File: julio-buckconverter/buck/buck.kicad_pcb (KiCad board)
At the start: 2 copper layers, 63.5 x 95.5 mm, 27 parts, among them J1 Screw_Terminal_01x02, J2 Screw_Terminal_01x02, J3 Screw_Terminal_01x02, Q1 BD911, Q2 MJE15031, U2 TL494

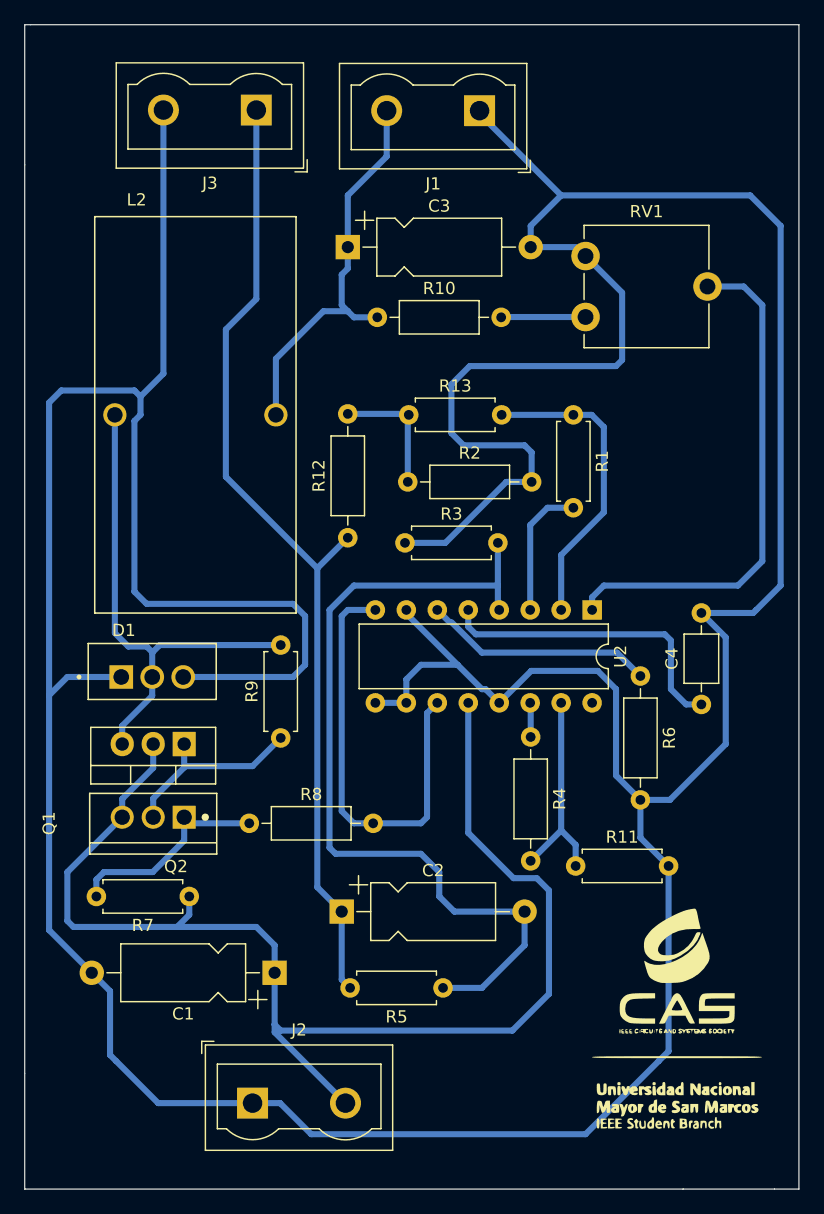
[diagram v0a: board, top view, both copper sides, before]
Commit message: CASI FINAL
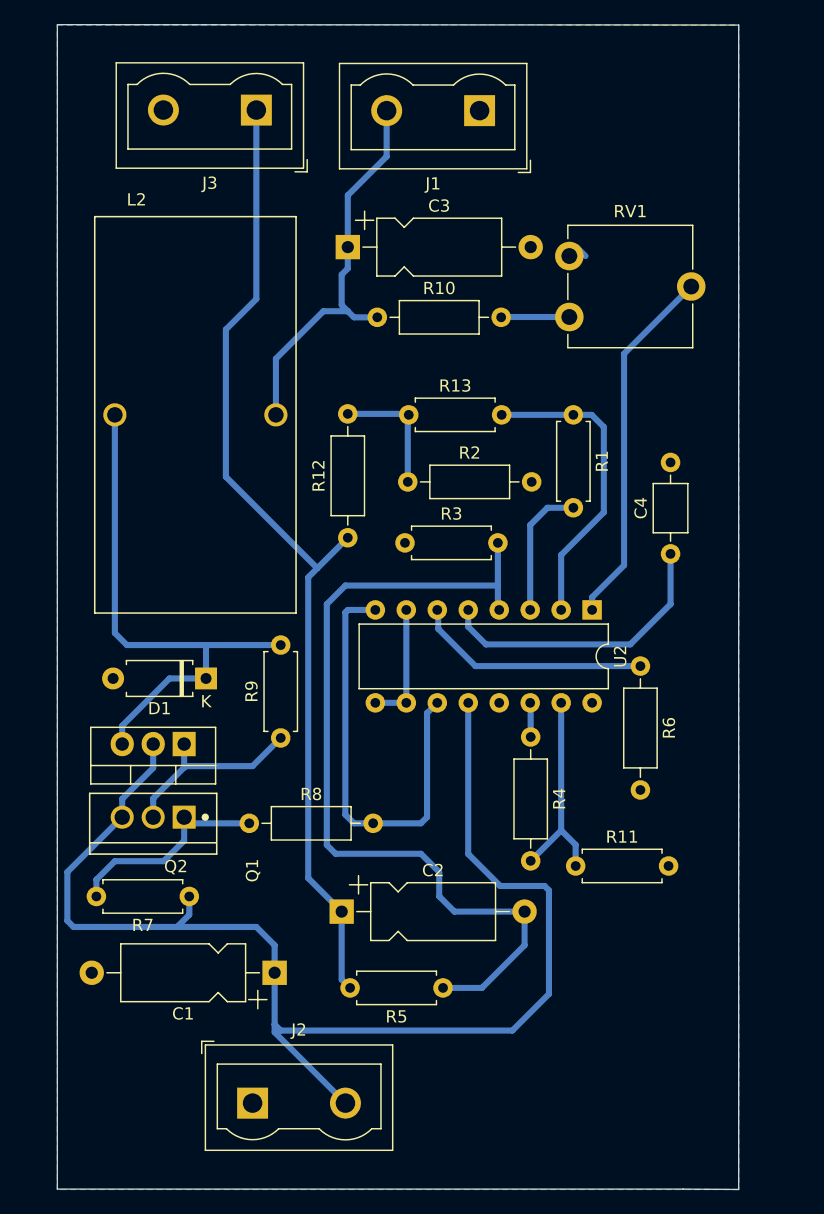
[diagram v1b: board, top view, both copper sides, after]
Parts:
- removed G***: LOGO, Image:Cas_logo_fin
- D1: value SR1050 -> D_Schottky; footprint SR1050:TO254P1050X476X2020-3 -> Diode_THT:D_A-405_P7.62mm_Horizontal
- moved C4 12.6 mm to (157.0, 76.9)
- moved D1 4.45 mm to (118.9, 87.1), turned to 180 degrees
- moved RV1 1.33 mm to (148.7, 57.5)
- moved R6 0.81 mm to (154.5, 86.1)
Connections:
- D1 pad 1: GND -> Net-(D1-K)
- D1 pad 2: Net-(Q1-E) -> GND
- L2 pad 1: Net-(Q1-E) -> Net-(D1-K)
- Q1 pad 3: Net-(Q1-E) -> Net-(D1-K)
- R9 pad 2: Net-(Q1-E) -> Net-(D1-K)
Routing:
- net GND: track 401.7 -> 12.0 mm
- net Net-(D1-K): track 0.00 -> 44.6 mm
- net Net-(Q1-E): track 41.0 -> 0.00 mm
- net 1in: track 42.4 -> 29.9 mm
- net Net-(U2-CT): track 25.5 -> 24.1 mm
- net Net-(R10-Pad2): track 6.93 -> 5.60 mm
- net Vin: track 105.2 -> 106.2 mm
- net 5v: track 80.8 -> 81.4 mm
- net Net-(U2-DTC): track 69.9 -> 70.5 mm
- net Net-(U2-RT): track 18.9 -> 19.4 mm
- added copper zone on B.Cu, net GND
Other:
- board size 63.5 x 95.5 mm -> 55.9 x 95.5 mm
- board text removed: "Buck Converter Circuit"
